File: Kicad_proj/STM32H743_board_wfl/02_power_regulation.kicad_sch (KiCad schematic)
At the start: 2 parts, among them U1 LT8609SEV#PBF, U2 TPS7A2033PDBVR

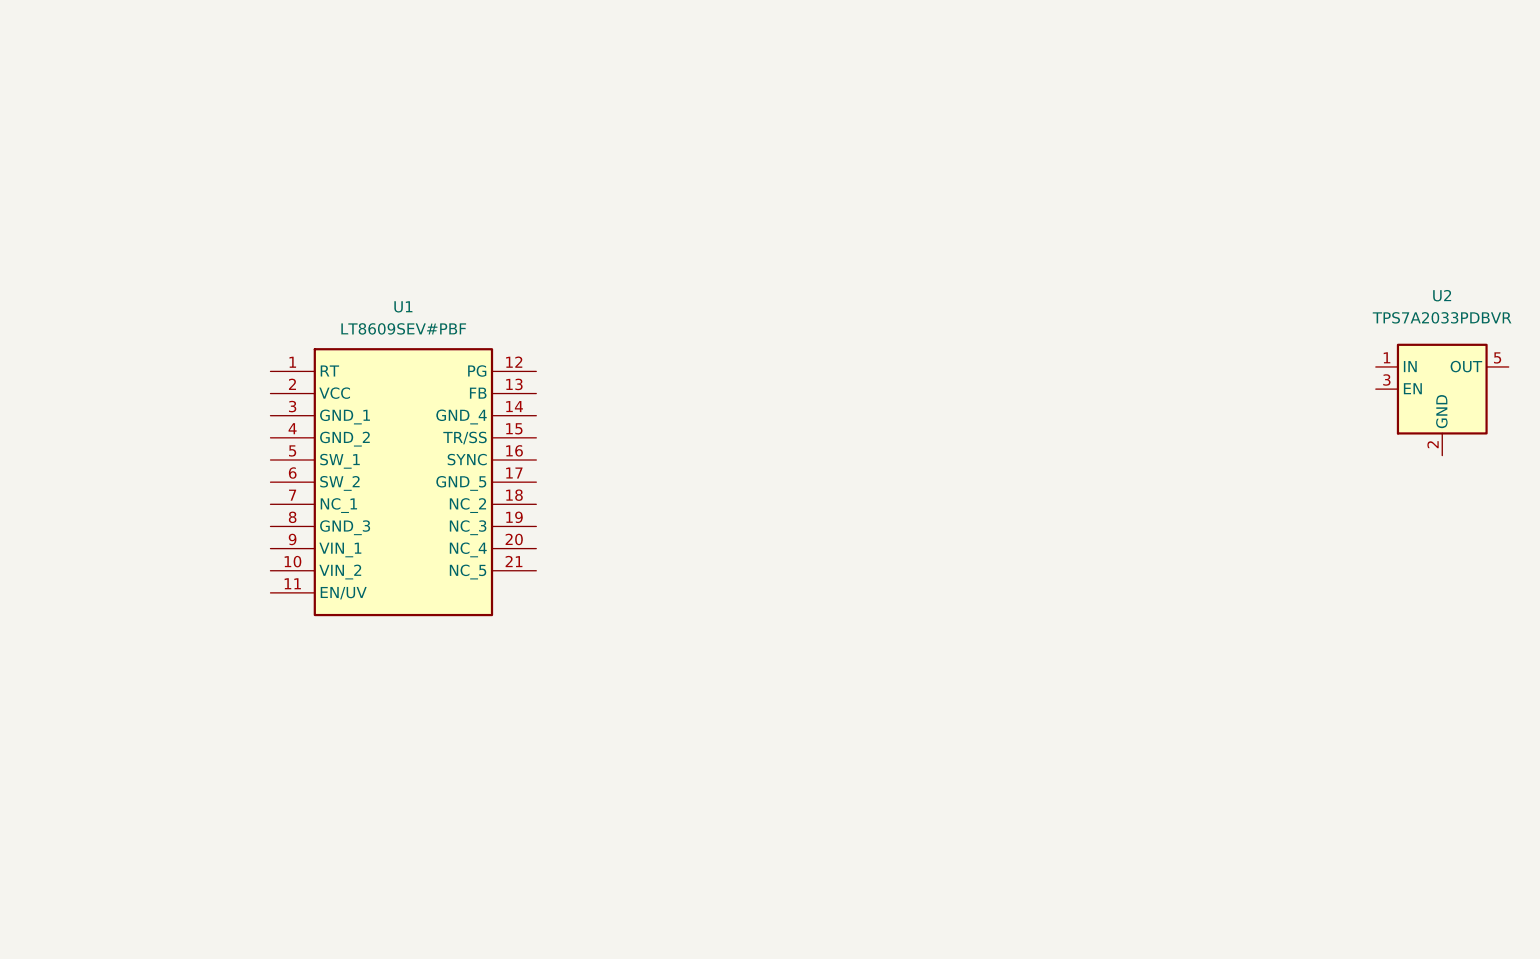
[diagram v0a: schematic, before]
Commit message: v0.4b power smps
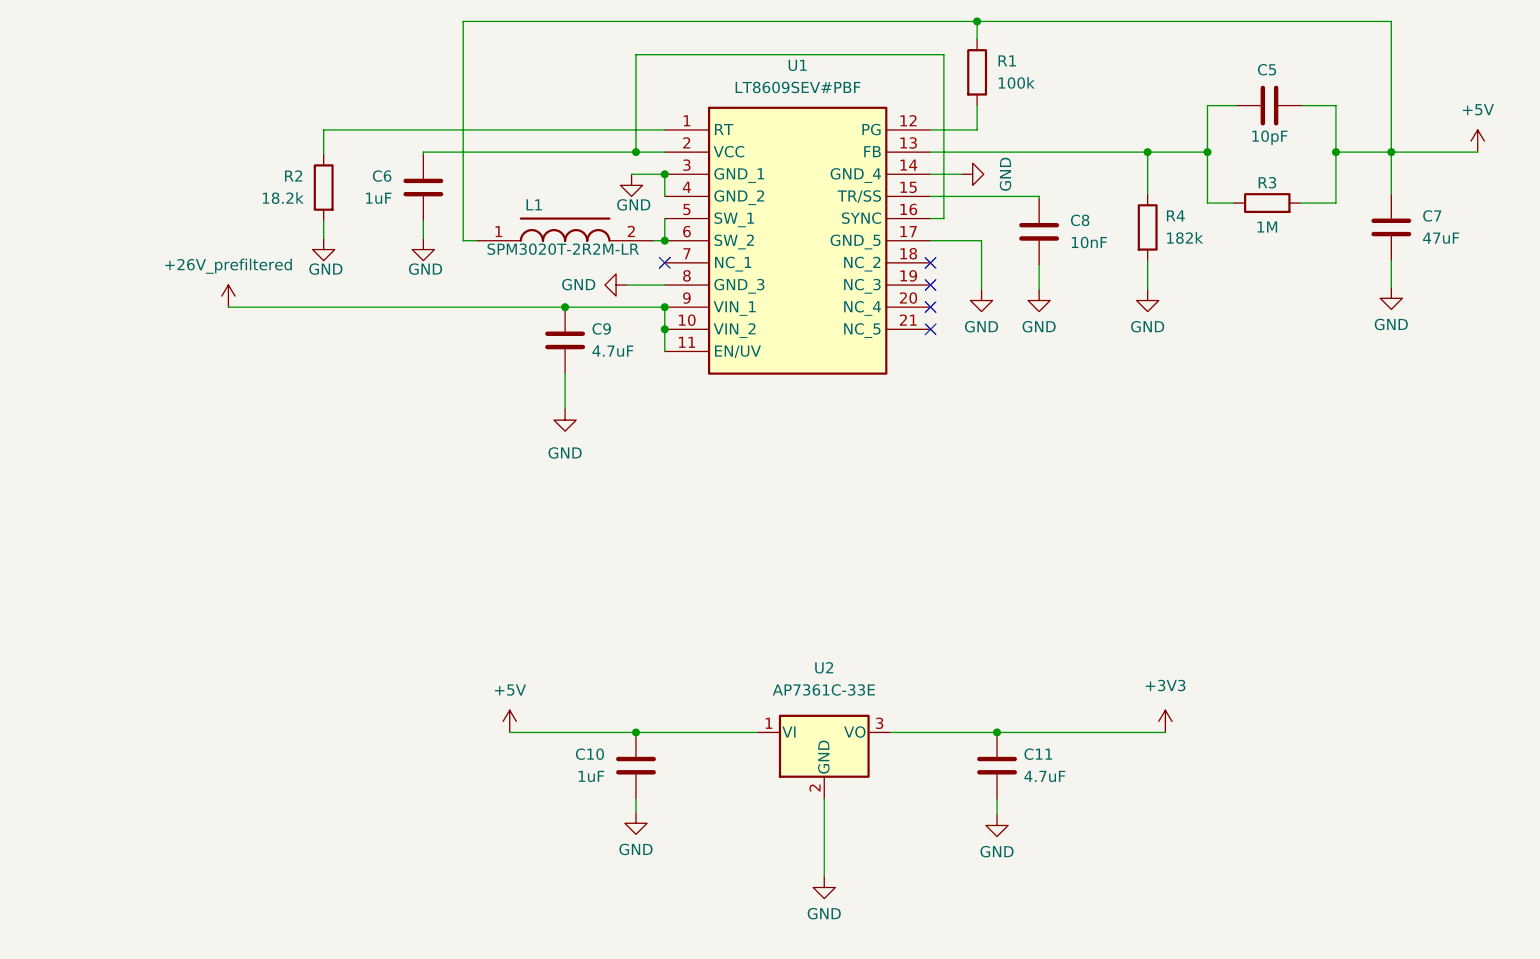
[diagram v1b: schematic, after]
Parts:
- removed U2: TPS7A2033PDBVR, Package_TO_SOT_SMD:SOT-23-5, symbol Regulator_Linear:TPS7A20xxxDBV
- added C10, C6: 1uF, Capacitor_SMD:C_0603_1608Metric, symbol Device:C
- added C11, C9: 4.7uF, Capacitor_SMD:C_0603_1608Metric, symbol Device:C
- added C5: 10pF, Capacitor_SMD:C_01005_0402Metric, symbol Device:C
- added C7: 47uF, Capacitor_SMD:C_1206_3216Metric, symbol Device:C
- added C8: 10nF, Capacitor_SMD:C_01005_0402Metric, symbol Device:C
- added L1: SPM3020T-2R2M-LR, STM32H743_board_library_footprints:SPM3010-3020, symbol STM32H743_board_library_symbols:SPM3020T-2R2M-LR
- added R1: 100k, Resistor_SMD:R_01005_0402Metric, symbol Device:R
- added R2: 18.2k, Resistor_SMD:R_01005_0402Metric, symbol Device:R
- added R3: 1M, Resistor_SMD:R_01005_0402Metric, symbol Device:R
- added R4: 182k, Resistor_SMD:R_01005_0402Metric, symbol Device:R
- added U2: AP7361C-33E, Package_TO_SOT_SMD:SOT-223-3_TabPin2, symbol Regulator_Linear:AP7361C-33E
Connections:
- net at U1.1 (RT): now also R2.1
- net +26V_prefiltered: now reaches U1.10 (VIN_2)
- net +26V_prefiltered: now also U1.11 (EN/UV), U1.9 (VIN_1), C9.1
- net at U1.12 (PG): now also R1.2
- net at U1.13 (FB): now also C5.1, R3.1, R4.1
- net GND: now reaches U1.14 (GND_4)
- net GND: now also U1.17 (GND_5), U1.3 (GND_1), U1.4 (GND_2), U1.8 (GND_3), C10.2, C11.2, C6.2, C7.2, C8.2, C9.2, R2.2, R4.2, U2.2 (GND)
- net at U1.15 (TR/SS): now also C8.1
- net at U1.16 (SYNC): now also U1.2 (VCC), C6.1
- net at U1.5 (SW_1): now also U1.6 (SW_2), L1.2
- new net +3V3: C11.1, U2.3 (VO)
- new net +5V: C10.1, C5.2, C7.1, L1.1, R1.1, R3.2, U2.1 (VI)
- no-connect marks 0 -> 5

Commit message: v0.5 schematics + lib update
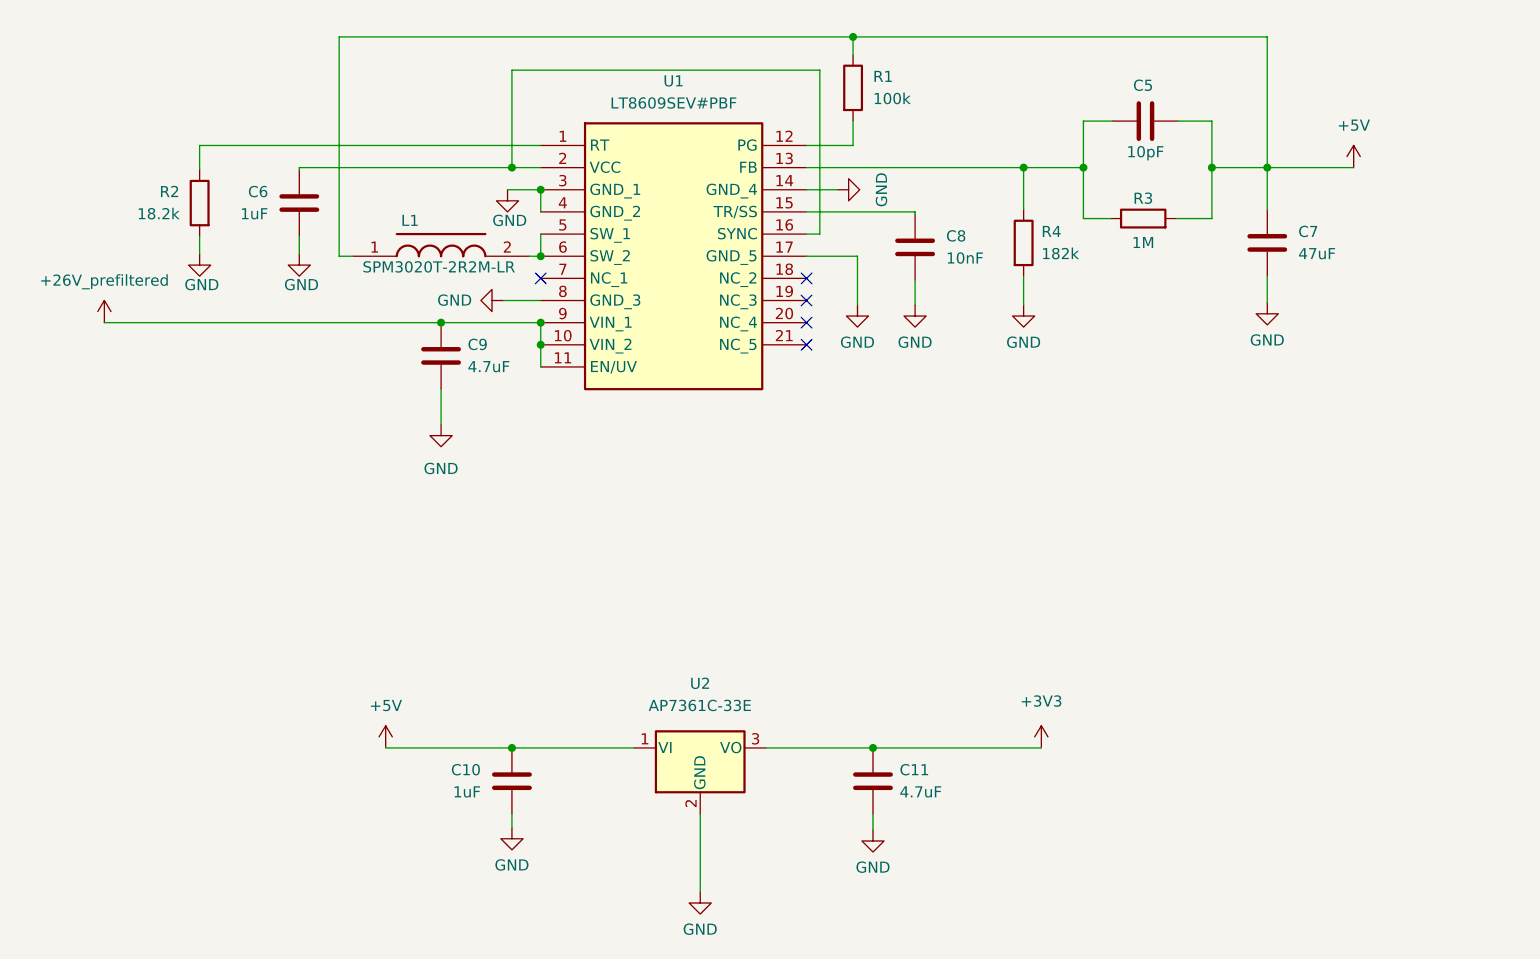
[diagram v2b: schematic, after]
